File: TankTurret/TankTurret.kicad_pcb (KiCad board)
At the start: 2 copper layers, 35 x 60 mm, 84 parts, among them J1 Conn_01x04_Socket, J2 USB_C_Receptacle_USB2.0_16P, J3 Conn_01x02, J4 Conn_01x02, J5 Conn_01x02, J6 Conn_01x03, Q1 MMBT3904, SW1 SW_Push, SW2 SW_Push, U1 ESP32-S3-WROOM-1, U3 ME6211C28M5G, U4 LN1234B132MR-G

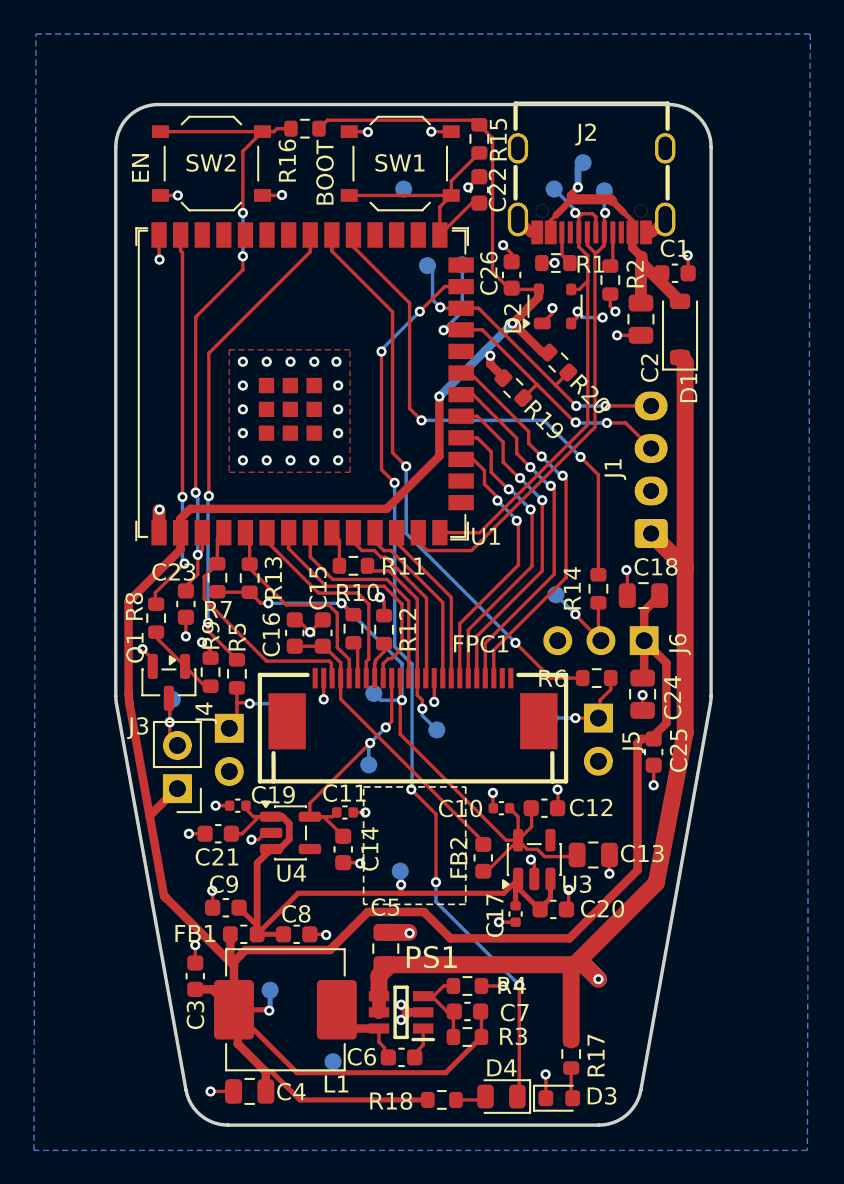
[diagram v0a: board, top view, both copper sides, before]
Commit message: Signed-off-by: SMAUG\Pete <pwbrophy@gmail.com>
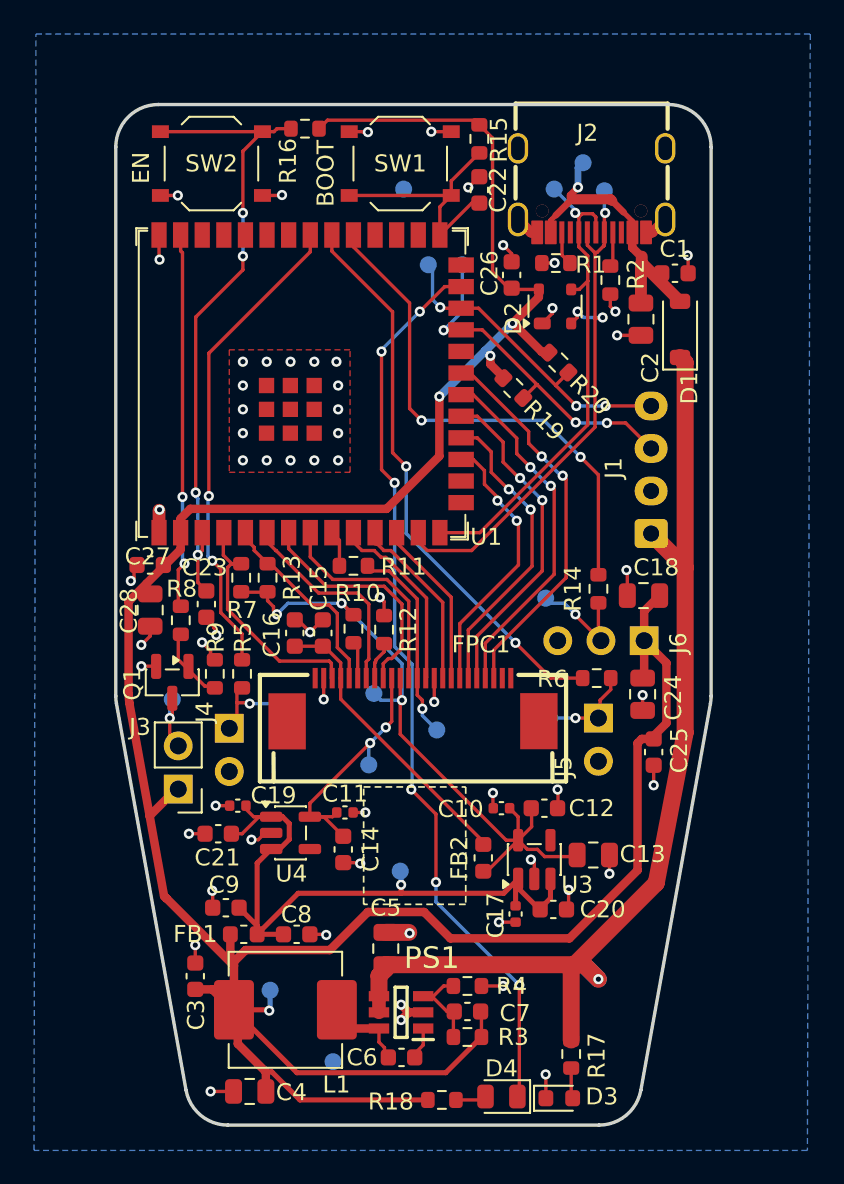
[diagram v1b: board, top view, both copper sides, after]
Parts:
- added C27: 100nF, Capacitor_SMD:C_0603_1608Metric, F.Cu at (55.9, 68.3)
- added C28: 10uF, Capacitor_SMD:C_0805_2012Metric, F.Cu at (55.9, 71.0)
- moved R8 1.46 mm to (57.6, 71.6)
- moved R7 1.40 mm to (61.2, 69.1)
- moved C23 1.20 mm to (59.1, 70.7)
- moved R13 1.05 mm to (62.8, 69.1)
- moved TP16 0.63 mm to (79.1, 70.3)
- moved R5 0.30 mm to (61.2, 74.8)
- moved R9 0.27 mm to (59.6, 74.8)
- moved Q1 0.20 mm to (57.1, 75.2)
- moved TP11 0.07 mm to (72.2, 50.7)
- moved J3 0.06 mm to (57.5, 81.5)
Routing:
- net GND: track 53.5 -> 55.5 mm, vias 59 -> 61
- net /GPIO5: track 12.5 -> 11.8 mm
- net Net-(Q1-B): track 4.74 -> 4.03 mm
- net Net-(J6-Pin_2): track 6.08 -> 6.60 mm
